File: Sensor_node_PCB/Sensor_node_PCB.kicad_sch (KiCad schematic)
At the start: 21 parts, among them J1 Conn_02x14_Counter_Clockwise, Q1 NMOS, Q2 NMOS, Q3 NMOS, U1 INA219AxD

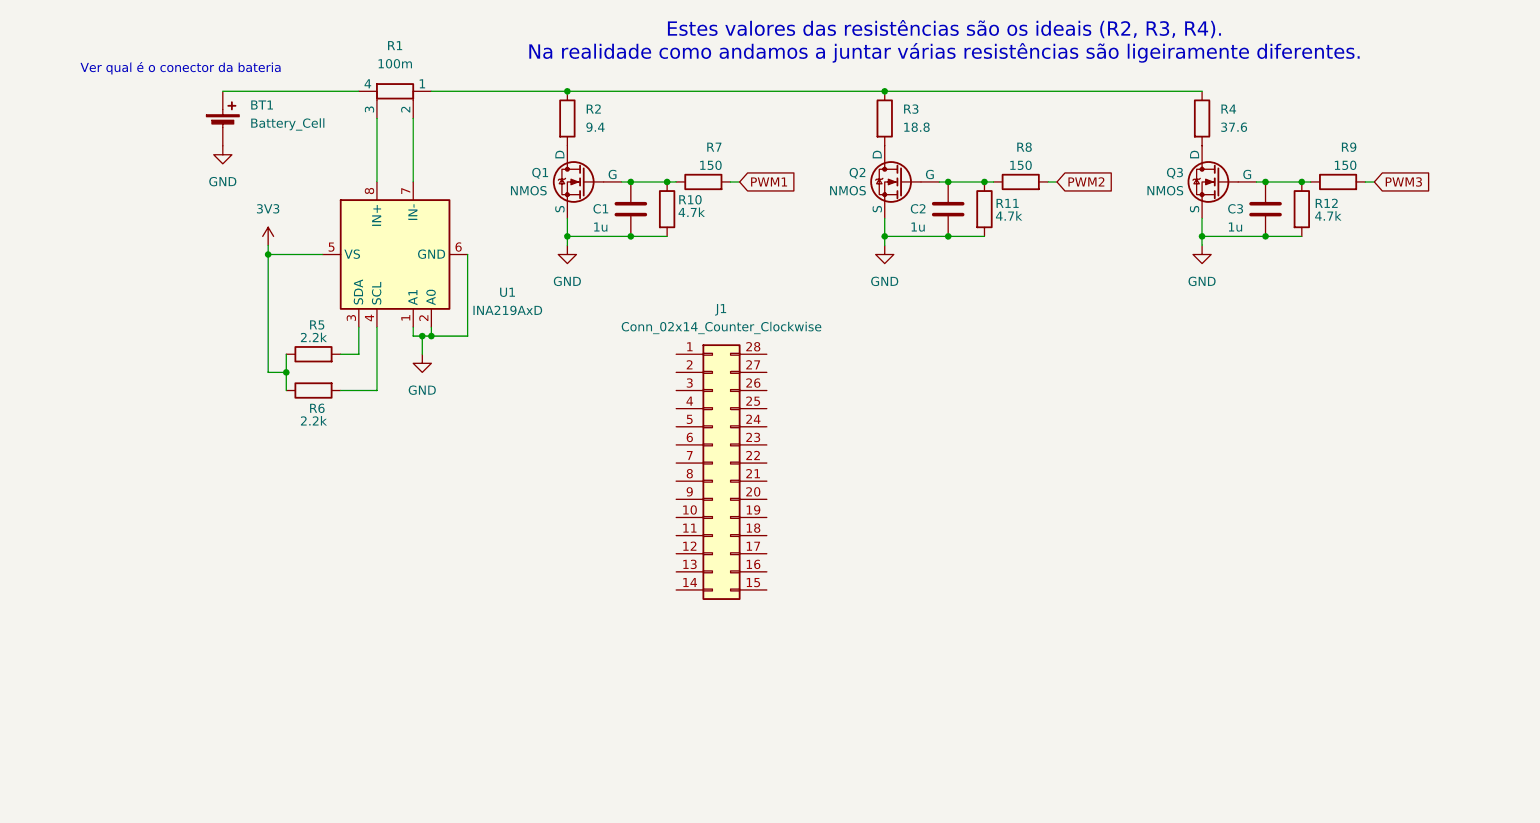
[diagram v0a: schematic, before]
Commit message: Node pcb schematic update
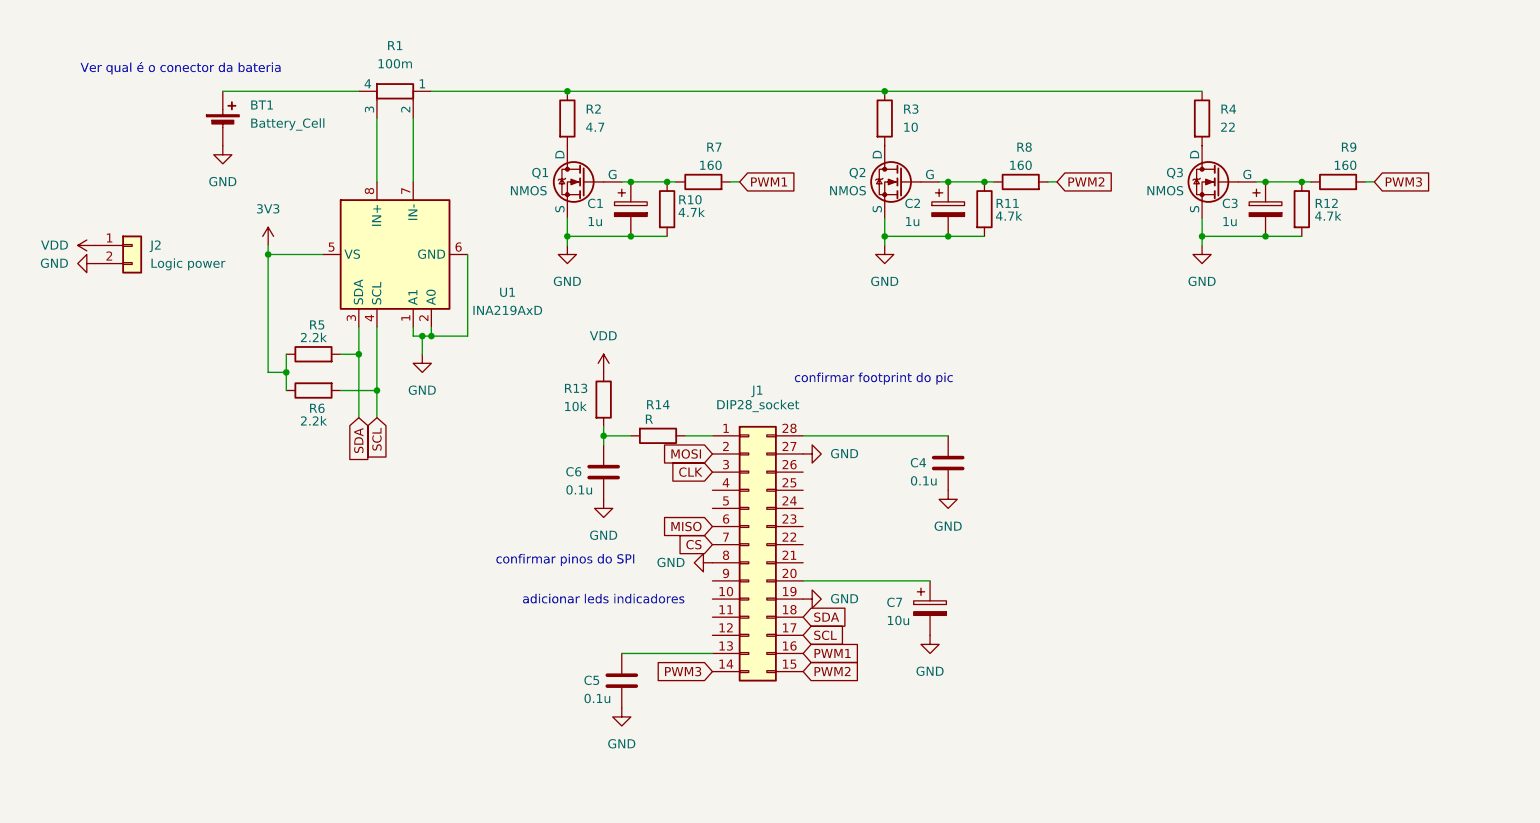
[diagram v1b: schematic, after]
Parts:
- removed C1, C2, C3: 1u, symbol Device:C
- added C1, C2, C3: 1u, symbol Device:C_Polarized
- added C4, C5, C6: 0.1u, symbol Device:C
- added C7: 10u, symbol Device:C_Polarized
- added J2: Logic power, symbol Connector_Generic:Conn_01x02
- added R13: 10k, symbol Device:R
- added R14: R, symbol Device:R
- J1: value Conn_02x14_Counter_Clockwise -> DIP28_socket; footprint (none) -> Package_DIP:DIP-28_W7.62mm_Socket
- R2: value 9.4 -> 4.7
- R3: value 18.8 -> 10
- R4: value 37.6 -> 22
- R7, R8, R9: value 150 -> 160
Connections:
- net GND: now also J1.19 (Pin_19), J1.27 (Pin_27), J1.8 (Pin_8), C1.2, C2.2, C3.2, C4.2, C5.2, C6.2, C7.2, J2.2 (Pin_2)
- net PWM1: now also J1.16 (Pin_16)
- net PWM2: now also J1.15 (Pin_15)
- net PWM3: now also J1.14 (Pin_14)
- net at J1.1 (Pin_1): now also R14.1
- net at J1.13 (Pin_13): now also C5.1
- net SCL: now reaches J1.17 (Pin_17)
- net SCL: now also R6.2, U1.4 (SCL)
- net SDA: now reaches J1.18 (Pin_18)
- net SDA: now also R5.2, U1.3 (SDA)
- net MOSI: now reaches J1.2 (Pin_2)
- net at J1.20 (Pin_20): now also C7.1
- net at J1.28 (Pin_28): now also C4.1
- net CLK: now reaches J1.3 (Pin_3)
- net MISO: now reaches J1.6 (Pin_6)
- net CS: now reaches J1.7 (Pin_7)
- net at Q2.2 (G), R11.1, R8.1: now also C2.1
- net at Q3.2 (G), R12.1, R9.1: now also C3.1
- net at Q1.2 (G), R10.1, R7.1: now also C1.1
- new net: C6.1, R13.2, R14.2
- new net VDD: J2.1 (Pin_1), R13.1
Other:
- note added: "adicionar leds indicadores"
- note added: "confirmar footprint do pic"
- note added: "confirmar pinos do SPI"
- note removed: "Estes valores das resistências são os ideais (R2, R3, R4). Na realidade como andamos a juntar várias resistências são ligeiramente diferentes."
- moved on the sheet: J1

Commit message: PCB schematic updates
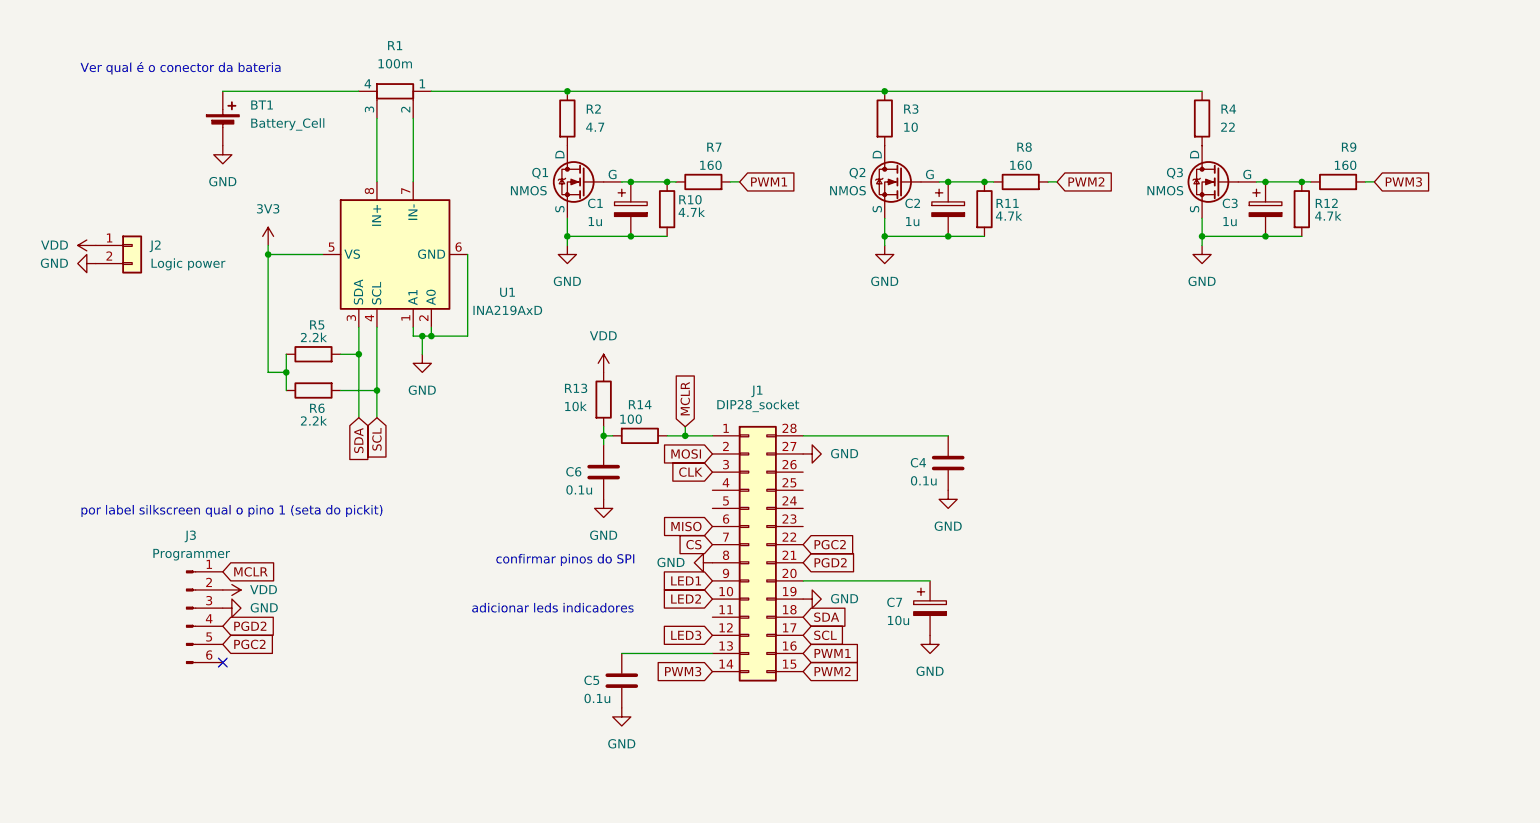
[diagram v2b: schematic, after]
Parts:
- added J3: Programmer, Connector_PinHeader_2.54mm:PinHeader_1x06_P2.54mm_Vertical, symbol Connector:Conn_01x06_Pin
- R14: value R -> 100
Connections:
- net GND: now also J3.3 (Pin_3)
- net VDD: now also J3.2 (Pin_2)
- net MCLR: now reaches J1.1 (Pin_1), R14.1
- net MCLR: now also J3.1 (Pin_1)
- net LED2: now reaches J1.10 (Pin_10)
- net LED3: now reaches J1.12 (Pin_12)
- net PGD2: now reaches J1.21 (Pin_21)
- net PGD2: now also J3.4 (Pin_4)
- net PGC2: now reaches J1.22 (Pin_22)
- net PGC2: now also J3.5 (Pin_5)
- net LED1: now reaches J1.9 (Pin_9)
- no-connect marks 0 -> 1
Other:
- note added: "por label silkscreen qual o pino 1 (seta do pickit)"
- note removed: "confirmar footprint do pic"
- moved on the sheet: R14

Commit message: PCB layout started
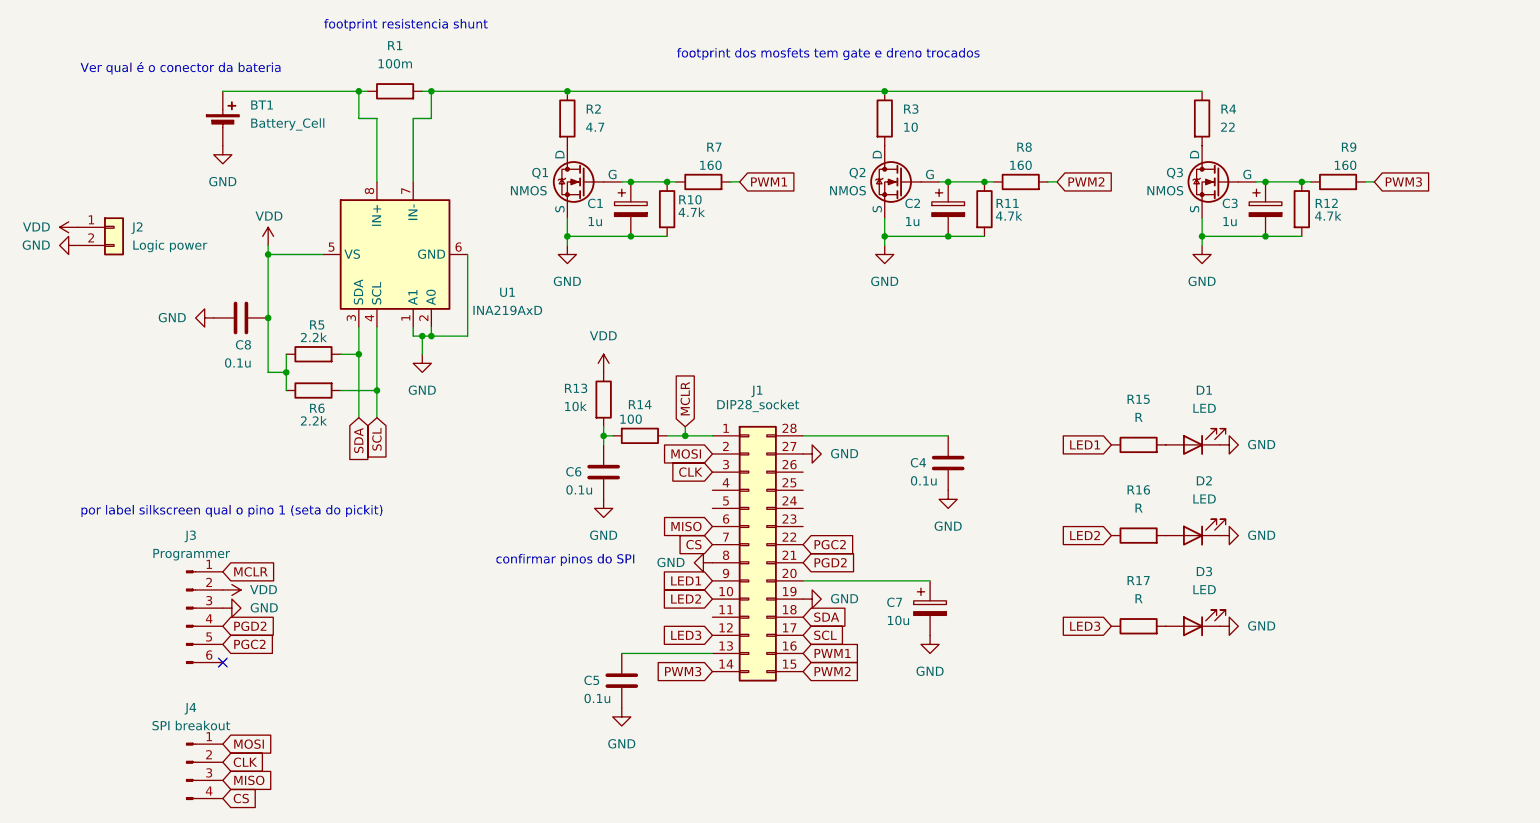
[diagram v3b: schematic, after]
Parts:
- removed R1: 100m, symbol Device:R_Shunt
- added C8: 0.1u, Capacitor_THT:C_Rect_L7.0mm_W3.5mm_P5.00mm, symbol Device:C
- added D1, D2, D3: LED, LED_THT:LED_D4.0mm, symbol Device:LED
- added J4: SPI breakout, Connector_PinHeader_2.54mm:PinHeader_1x04_P2.54mm_Vertical, symbol Connector:Conn_01x04_Pin
- added R1: 100m, Resistor_THT:R_Axial_DIN0309_L9.0mm_D3.2mm_P12.70mm_Horizontal, symbol Device:R
- added R15, R16, R17: R, Resistor_THT:R_Axial_DIN0309_L9.0mm_D3.2mm_P12.70mm_Horizontal, symbol Device:R
- BT1: footprint (none) -> Connector_PinHeader_1.00mm:PinHeader_1x02_P1.00mm_Vertical
- C1, C2, C3, C7: footprint (none) -> Capacitor_THT:CP_Radial_D5.0mm_P2.00mm
- C4, C5, C6: footprint (none) -> Capacitor_THT:C_Rect_L7.0mm_W3.5mm_P5.00mm
- J2: footprint (none) -> Connector_PinHeader_2.54mm:PinHeader_1x02_P2.54mm_Vertical
- Q1, Q2, Q3: footprint (none) -> Package_TO_SOT_THT:TO-220-3_Vertical
- R10, R11, R12, R13, R14, R5, R6, R7, R8, R9: footprint (none) -> Resistor_THT:R_Axial_DIN0309_L9.0mm_D3.2mm_P12.70mm_Horizontal
- R2: footprint (none) -> Resistor_THT:R_Axial_Power_L38.0mm_W9.0mm_P45.72mm
- R3, R4: footprint (none) -> Resistor_THT:R_Axial_Power_L50.0mm_W9.0mm_P55.88mm
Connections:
- net 3V3 is gone; now on net VDD: R5.1, R6.1, U1.5 (VS)
- net CLK: now also J4.2 (Pin_2)
- net CS: now also J4.4 (Pin_4)
- net GND: now also C8.1, D1.1 (K), D2.1 (K), D3.1 (K)
- net LED1: now also R15.1
- net LED2: now also R16.1
- net LED3: now also R17.1
- net MISO: now also J4.3 (Pin_3)
- net MOSI: now also J4.1 (Pin_1)
- net VDD: now also C8.2
- net at R2.1, R3.1, R4.1: now also U1.7 (IN-), R1.2
- net at U1.8 (IN+): now also BT1.1 (+), R1.1
- new net: D2.2 (A), R16.2
- new net: D1.2 (A), R15.2
- new net: D3.2 (A), R17.2
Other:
- note added: "footprint dos mosfets tem gate e dreno trocados"
- note added: "footprint resistencia shunt"
- note removed: "adicionar leds indicadores"
- moved on the sheet: J2

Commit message: PCB corrections and improvements
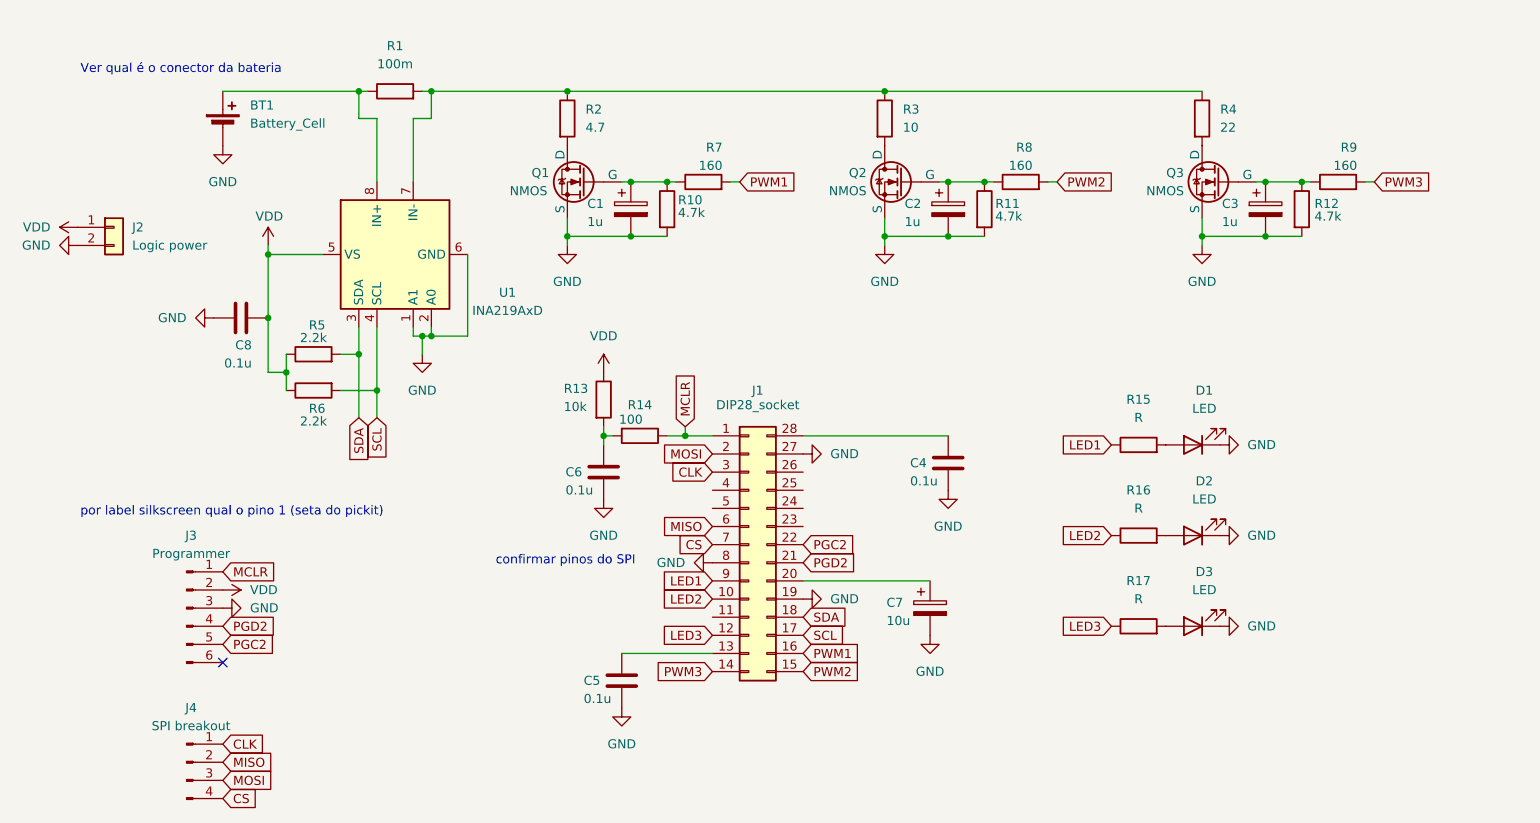
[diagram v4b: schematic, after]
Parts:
- Q1, Q2, Q3: footprint Package_TO_SOT_THT:TO-220-3_Vertical -> Package_TO_SOT_THT:TO-220F-3_Horizontal_TabUp
- R1: footprint Resistor_THT:R_Axial_DIN0309_L9.0mm_D3.2mm_P12.70mm_Horizontal -> Capacitor_SMD:C_1206_3216Metric_Pad1.33x1.80mm_HandSolder
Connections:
- net CLK: now also J4.1 (Pin_1); no longer J4.2 (Pin_2)
- net MISO: now also J4.2 (Pin_2); no longer J4.3 (Pin_3)
- net MOSI: now also J4.3 (Pin_3); no longer J4.1 (Pin_1)
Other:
- note removed: "footprint dos mosfets tem gate e dreno trocados"
- note removed: "footprint resistencia shunt"
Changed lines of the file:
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@@
 		)
 	)
-	(text "footprint resistencia shunt"
-		(exclude_from_sim no)
-		(at 72.644 16.256 0)
-		(effects
-			(font
-				(size 1.27 1.27)
-			)
-		)
-	)
-	(text "footprint dos mosfets tem gate e dreno trocados"
-		(exclude_from_sim no)
-		(at 131.826 20.32 0)
-		(effects
-			(font
-				(size 1.27 1.27)
-			)
-		)
-	)
 	(global_label "PGC2"
 		(shape input)
@@
 		)
 	)
+	(global_label "CLK"
+		(shape input)
+		(at 46.99 116.84 0)
+		(fields_autoplaced yes)
+		(effects
+			(font
+				(size 1.27 1.27)
+			)
+			(justify left)
+		)
+		(property "Intersheetrefs" "${INTERSHEET_REFS}"
+			(at 53.5433 116.84 0)
+			(effects
+				(font
+					(size 1.27 1.27)
+				)
+				(justify left)
+				(hide yes)
+			)
+		)
+	)
 	(global_label "PGC2"
 		(shape input)
@@
 		)
 	)
-	(global_label "CLK"
+	(global_label "MOSI"
 		(shape input)
-		(at 115.57 78.74 180)
+		(at 46.99 121.92 0)
 		(fields_autoplaced yes)
 		(effects
@@
 				(size 1.27 1.27)
 			)
-			(justify right)
+			(justify left)
 		)
 		(property "Intersheetrefs" "${INTERSHEET_REFS}"
-			(at 109.0167 78.74 0)
+			(at 54.5714 121.92 0)
 			(effects
 				(font
 					(size 1.27 1.27)
 				)
-				(justify right)
+				(justify left)
 				(hide yes)
 			)
 		)
 	)
-	(global_label "LED1"
+	(global_label "CLK"
 		(shape input)
-		(at 171.45 74.93 180)
+		(at 115.57 78.74 180)
 		(fields_autoplaced yes)
 		(effects
@@
 		)
 		(property "Intersheetrefs" "${INTERSHEET_REFS}"
-			(at 163.8082 74.93 0)
+			(at 109.0167 78.74 0)
 			(effects
 				(font
@@
 		)
 	)
-	(global_label "CS"
+	(global_label "LED1"
 		(shape input)
-		(at 115.57 88.9 180)
+		(at 171.45 74.93 180)
 		(fields_autoplaced yes)
 		(effects
@@
 		)
 		(property "Intersheetrefs" "${INTERSHEET_REFS}"
-			(at 110.1053 88.9 0)
+			(at 163.8082 74.93 0)
 			(effects
 				(font
@@
 		)
 	)
-	(global_label "SDA"
+	(global_label "CS"
 		(shape input)
-		(at 128.27 99.06 0)
+		(at 115.57 88.9 180)
 		(fields_autoplaced yes)
 		(effects
@@
 				(size 1.27 1.27)
 			)
-			(justify left)
+			(justify right)
 		)
 		(property "Intersheetrefs" "${INTERSHEET_REFS}"
-			(at 134.8233 99.06 0)
+			(at 110.1053 88.9 0)
 			(effects
 				(font
 					(size 1.27 1.27)
 				)
-				(justify left)
+				(justify right)
 				(hide yes)
 			)
 		)
 	)
-	(global_label "CLK"
+	(global_label "SDA"
 		(shape input)
-		(at 46.99 119.38 0)
+		(at 128.27 99.06 0)
 		(fields_autoplaced yes)
 		(effects
@@
 		)
 		(property "Intersheetrefs" "${INTERSHEET_REFS}"
-			(at 53.5433 119.38 0)
+			(at 134.8233 99.06 0)
 			(effects
 				(font
@@
 		)
 	)
-	(global_label "MOSI"
-		(shape input)
-		(at 46.99 116.84 0)
-		(fields_autoplaced yes)
-		(effects
-			(font
-				(size 1.27 1.27)
-			)
-			(justify left)
-		)
-		(property "Intersheetrefs" "${INTERSHEET_REFS}"
-			(at 54.5714 116.84 0)
-			(effects
-				(font
-					(size 1.27 1.27)
-				)
-				(justify left)
-				(hide yes)
-			)
-		)
-	)
 	(global_label "LED3"
 		(shape input)
@@
 	(global_label "MISO"
 		(shape input)
-		(at 46.99 121.92 0)
+		(at 46.99 119.38 0)
 		(fields_autoplaced yes)
 		(effects
@@
 		)
 		(property "Intersheetrefs" "${INTERSHEET_REFS}"
-			(at 54.5714 121.92 0)
+			(at 54.5714 119.38 0)
 			(effects
 				(font
@@
 			)
 		)
-		(property "Footprint" "Resistor_THT:R_Axial_DIN0309_L9.0mm_D3.2mm_P12.70mm_Horizontal"
+		(property "Footprint" "Capacitor_SMD:C_1206_3216Metric_Pad1.33x1.80mm_HandSolder"
 			(at 71.12 27.178 90)
 			(effects
@@
 			)
 		)
-		(property "Footprint" "Package_TO_SOT_THT:TO-220-3_Vertical"
+		(property "Footprint" "Package_TO_SOT_THT:TO-220F-3_Horizontal_TabUp"
 			(at 181.61 35.56 0)
 			(effects
@@
 			)
 		)
-		(property "Footprint" "Package_TO_SOT_THT:TO-220-3_Vertical"
+		(property "Footprint" "Package_TO_SOT_THT:TO-220F-3_Horizontal_TabUp"
 			(at 137.16 35.56 0)
 			(effects
@@
 			)
 		)
-		(property "Footprint" "Package_TO_SOT_THT:TO-220-3_Vertical"
+		(property "Footprint" "Package_TO_SOT_THT:TO-220F-3_Horizontal_TabUp"
 			(at 92.71 35.56 0)
 			(effects
